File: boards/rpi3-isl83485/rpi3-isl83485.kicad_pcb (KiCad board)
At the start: 2 copper layers, 27.9 x 15.2 mm, 11 parts, among them J1 RPi, J2 JST-GH, U1 ISL83485

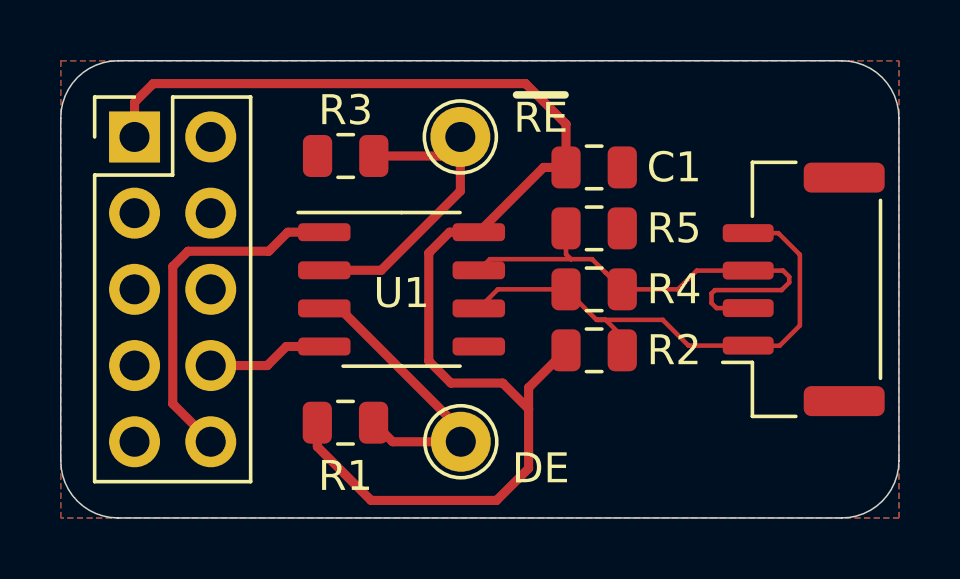
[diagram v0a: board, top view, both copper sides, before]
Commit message: Send to fab.
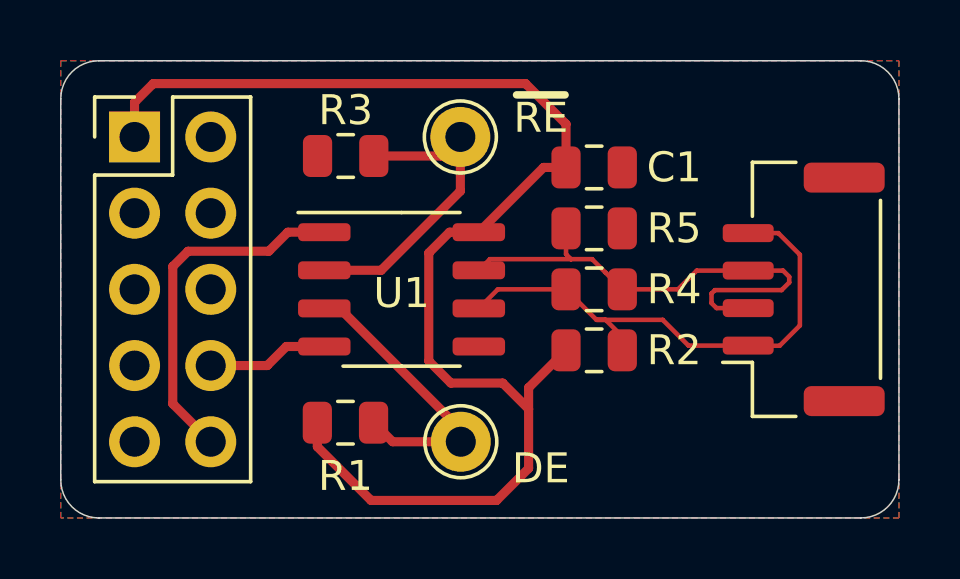
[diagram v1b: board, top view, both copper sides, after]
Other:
- outline, holes or cut-outs redrawn
- board text added: "rpi3<>isl83485 fourside.io"
- board text removed: "rpi3-isl83485 fourside.io"
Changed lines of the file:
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@@
   (page A4)
   (layers
-    (0 F.Cu signal)
-    (31 B.Cu signal)
+    (0 F.Cu signal hide)
+    (31 B.Cu signal hide)
     (32 B.Adhes user hide)
     (33 F.Adhes user hide)
@@
   )
   (setup
-    (last_trace_width 0.1524)
+    (last_trace_width 0.25)
     (user_trace_width 0.1016)
     (user_trace_width 0.1524)
@@
       (usegerberextensions false)
       (usegerberattributes false)
-      (usegerberadvancedattributes false)
+      (usegerberadvancedattributes true)
       (creategerberjobfile false)
-      (excludeedgelayer true)
-      (linewidth 0.100000)
+      (excludeedgelayer false)
+      (linewidth 0.150000)
       (plotframeref false)
       (viasonmask false)
       (mode 1)
-      (useauxorigin false)
+      (useauxorigin true)
       (hpglpennumber 1)
       (hpglpenspeed 20)
@@
       (psa4output false)
       (plotreference true)
-      (plotvalue true)
+      (plotvalue false)
       (plotinvisibletext false)
       (padsonsilk false)
-      (subtractmaskfromsilk false)
+      (subtractmaskfromsilk true)
       (outputformat 1)
       (mirror false)
-      (drillshape 1)
+      (drillshape 0)
       (scaleselection 1)
-      (outputdirectory ""))
+      (outputdirectory "gerbers/"))
   )
   (net 0 "")
@@
     (pad 8 smd roundrect (at 2.575 -1.905) (size 1.75 0.6) (layers F.Cu F.Paste F.Mask) (roundrect_rratio 0.25)
       (net 2 +3V3))
-    (model ${KISYS3DMOD}/Package_SO.3dshapes/SO-8_3.9x4.9mm_P1.27mm.wrl
+    (model ${KISYS3DMOD}/Package_SO.3dshapes/HSOP-8-1EP_3.9x4.9mm_P1.27mm_EP2.41x3.1mm.wrl
       (at (xyz 0 0 0))
       (scale (xyz 1 1 1))
@@
     )
   )
-  (gr_text "rpi3-isl83485\nfourside.io" (at 43.561 22.86) (layer B.Mask)
+  (gr_arc (start 43.18 29.21) (end 43.18 30.48) (angle -90) (layer Edge.Cuts) (width 0.05))
+  (gr_arc (start 17.78 29.21) (end 16.51 29.21) (angle -90) (layer Edge.Cuts) (width 0.05))
+  (gr_arc (start 17.78 16.51) (end 17.78 15.24) (angle -90) (layer Edge.Cuts) (width 0.05))
+  (gr_arc (start 43.18 16.51) (end 44.45 16.51) (angle -90) (layer Edge.Cuts) (width 0.05))
+  (gr_text "rpi3<>isl83485\nfourside.io" (at 43.561 22.86) (layer B.Mask)
     (effects (font (size 1.5 1.5) (thickness 0.3)) (justify left mirror))
   )
@@
     (effects (font (size 1 1) (thickness 0.25)))
   )
-  (gr_arc (start 18.415 28.575) (end 16.51 28.575) (angle -90) (layer Edge.Cuts) (width 0.05))
-  (gr_arc (start 18.415 17.145) (end 18.415 15.24) (angle -90) (layer Edge.Cuts) (width 0.05))
-  (gr_arc (start 42.545 28.575) (end 42.545 30.48) (angle -90) (layer Edge.Cuts) (width 0.05))
-  (gr_arc (start 42.545 17.145) (end 44.45 17.145) (angle -90) (layer Edge.Cuts) (width 0.05))
-  (gr_line (start 16.51 28.575) (end 16.51 17.145) (layer Edge.Cuts) (width 0.05))
-  (gr_line (start 42.545 30.48) (end 18.415 30.48) (layer Edge.Cuts) (width 0.05))
-  (gr_line (start 44.45 17.145) (end 44.45 28.575) (layer Edge.Cuts) (width 0.05))
-  (gr_line (start 18.415 15.24) (end 42.545 15.24) (layer Edge.Cuts) (width 0.05))
+  (gr_line (start 16.51 29.21) (end 16.51 16.51) (layer Edge.Cuts) (width 0.05))
+  (gr_line (start 43.18 30.48) (end 17.78 30.48) (layer Edge.Cuts) (width 0.05))
+  (gr_line (start 44.45 16.51) (end 44.45 29.21) (layer Edge.Cuts) (width 0.05))
+  (gr_line (start 17.78 15.24) (end 43.18 15.24) (layer Edge.Cuts) (width 0.05))
   (segment (start 29.47 20.955) (end 30.445 20.955) (width 0.3048) (layer F.Cu) (net 2))
   (segment (start 28.7782 21.6468) (end 29.47 20.955) (width 0.3048) (layer F.Cu) (net 2))
